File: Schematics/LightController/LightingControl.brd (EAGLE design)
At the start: 100 x 80 mm, 18 parts, among them IC1 LM324N, X2 87758-0816

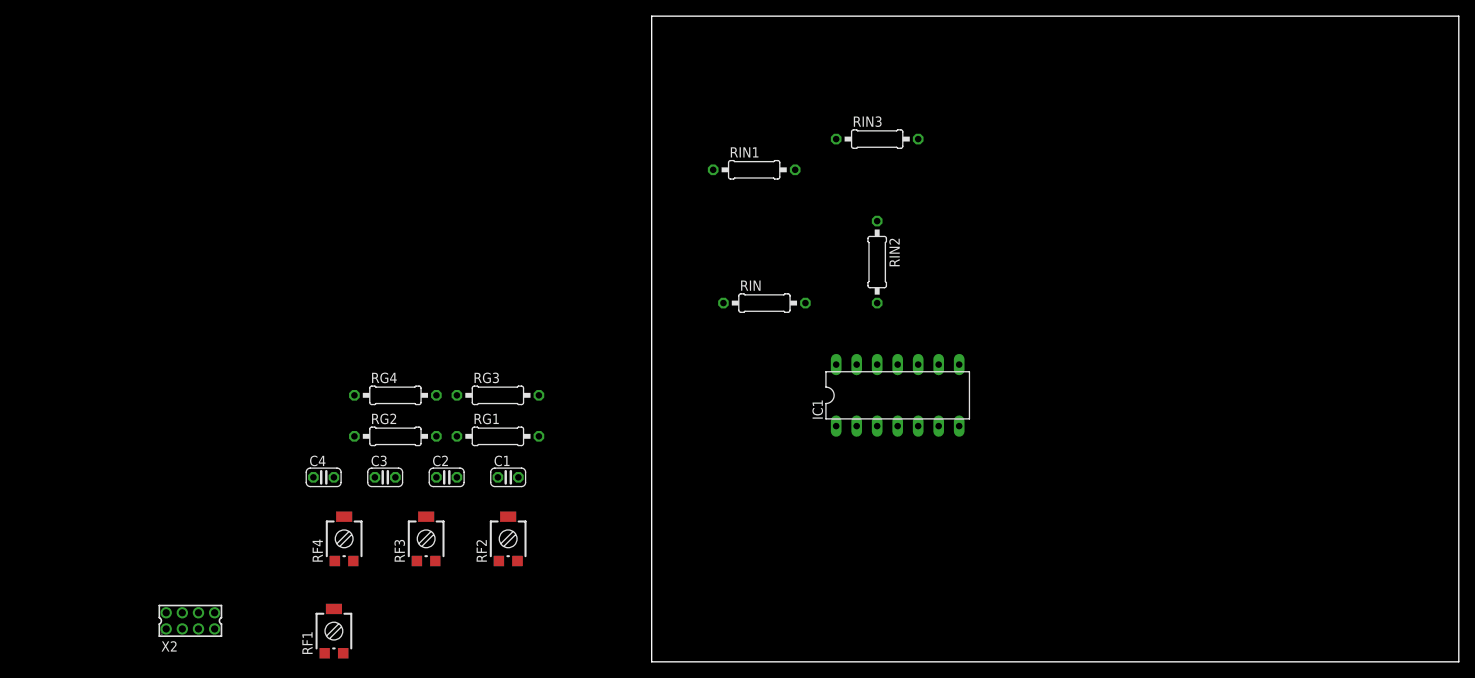
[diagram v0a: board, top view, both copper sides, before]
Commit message: updates to Light Schematics
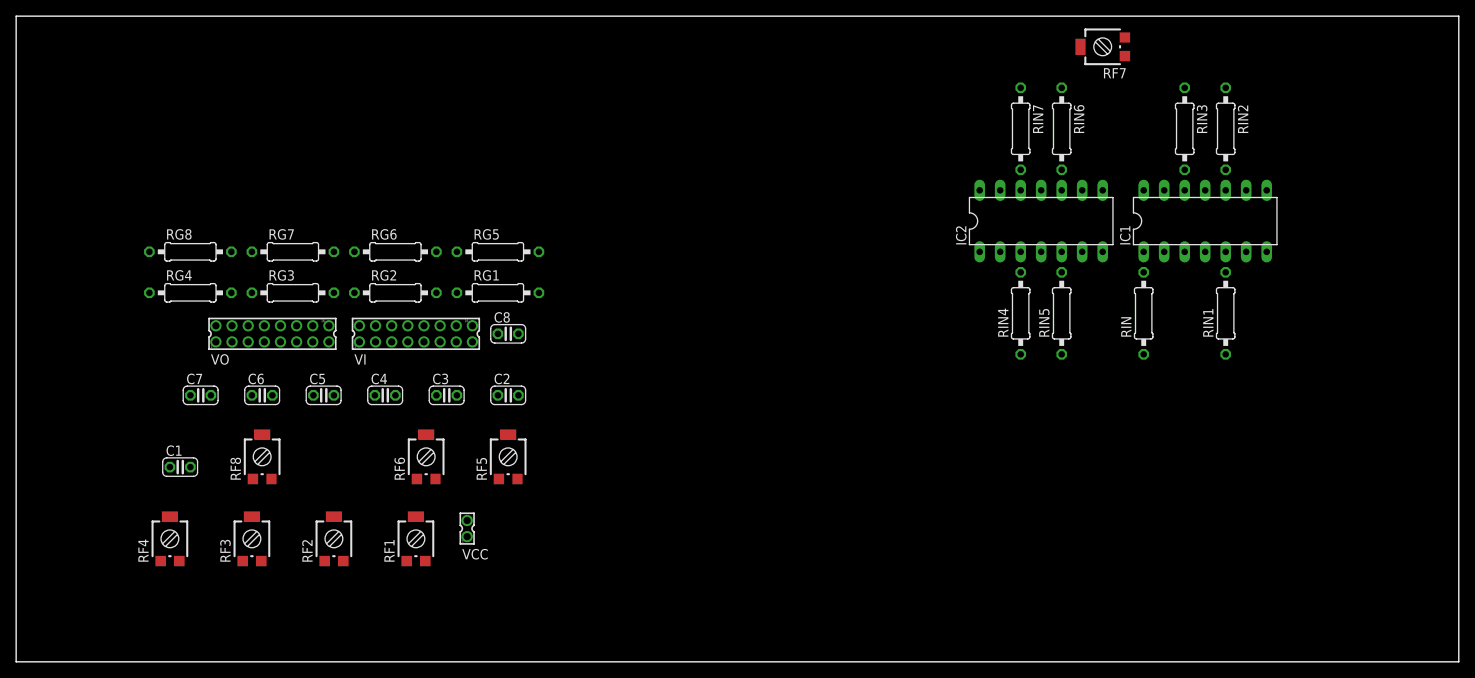
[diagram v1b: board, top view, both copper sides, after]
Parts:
- removed X2: 87758-0816, con-molex:87758-0816
- added C5, C6, C7, C8: 3300uF, rcl:C025-024X044
- added IC2: LM324N, linear:DIL14
- added RF5, RF6, RF7, RF8: 2M, rcl:RTRIM3314G
- added RG5, RG6, RG7, RG8: 1M, rcl:0207/10
- added RIN4, RIN5, RIN6, RIN7: (no value), rcl:0207/10
- added VCC: 87758-0216, con-molex:87758-0216
- added VI, VO: 87758-1616, con-molex:87758-1616
- moved RIN1 61.1 mm to (71.1, 43.2), turned to 90 degrees
- moved RIN 47.0 mm to (61.0, 43.2), turned to 90 degrees
- moved RIN2 46.2 mm to (71.1, 66.0)
- moved IC1 43.8 mm to (68.6, 54.6)
- moved C1 40.7 mm to (-58.4, 24.1)
- moved RIN3 38.1 mm to (66.0, 66.0), turned to 270 degrees
- moved RG3 28.4 mm to (-44.5, 45.7)
- moved RG4 28.4 mm to (-57.1, 45.7)
- moved RF3 21.6 mm to (-49.5, 15.2)
- moved RF2 21.6 mm to (-39.4, 15.2)
- moved RF4 21.6 mm to (-59.7, 15.2)
- moved RG1 17.8 mm to (-19.1, 45.7)
- moved RG2 17.8 mm to (-31.8, 45.7)
- moved RF1 15.3 mm to (-29.2, 15.2)
- moved C3 12.7 mm to (-25.4, 33.0)
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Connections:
- removed net V-: IC1.11
- removed net V03+: X2.5
- removed net V04+: X2.7
- removed net VI$1: C1.1, C2.1, C3.1, C4.1, RIN.1, RIN1.1, RIN2.1, RIN3.1
- new net N$10: IC2.3, RIN4.2
- new net N$11: IC2.6, RF6.2, RG6.2
- new net N$12: IC2.5, RIN5.2
- new net N$13: IC2.9, RF7.2, RG7.2
- new net N$14: IC2.13, RF8.2, RG8.2
- new net N$15: IC2.10, RIN6.2
- new net N$16: IC2.12, RIN7.2
- new net N$9: IC2.2, RF5.2, RG5.2
- new net VCC: VCC.1
- new net VI1: C1.1, RIN.1
- new net VI1+: VI.1
- new net VI2: C2.1, RIN1.1
- new net VI2+: VI.3
- new net VI3: C3.1, RIN2.1
- new net VI3+: VI.5
- new net VI4: C4.1, RIN3.1
- new net VI4+: VI.7
- new net VI5: C5.1, RIN4.1
- new net VI5+: VI.9
- new net VI6: C6.1, RIN5.1
- new net VI6+: VI.11
- new net VI7: C7.1, RIN6.1
- new net VI7+: VI.13
- new net VI8: C8.1, RIN7.1
- new net VI8+: VI.15
- new net VO5+: IC2.1, RF5.1, VO.9
- new net VO6+: IC2.7, RF6.1, VO.11
- new net VO7+: IC2.8, RF7.1, VO.13
- new net VO8+: IC2.14, RF8.1, VO.15
- net 0: now also C5.2, C6.2, C7.2, C8.2, RF5.3, RF6.3, RF7.3, RF8.3, RG5.1, RG6.1, RG7.1, RG8.1; no longer RG2.1
- net GND: now also IC1.11, IC2.11, RG2.1, VCC.2, VI.10, VI.12, VI.14, VI.16, VI.2, VI.4, VI.6, VI.8, VO.10, VO.12, VO.14, VO.16, VO.2, VO.4, VO.6, VO.8; no longer X2.2, X2.4, X2.6, X2.8
- net V+: now also IC2.4
- net VO1+: now also VO.1; no longer X2.1
- net VO2+: now also VO.3; no longer X2.3
- net VO3+: now also VO.5
- net VO4+: now also VO.7
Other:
- board size 100 x 80 mm -> 178.7 x 80 mm
